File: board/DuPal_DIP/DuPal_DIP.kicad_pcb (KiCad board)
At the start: 2 copper layers, 113 x 78.7 mm, 57 parts, among them J1 AVR-ISP-6, J2 RS232, J3 Power IN, SW1 SW_Push, SW2 Power, U1 ATmega8A-PU, U10 24 Pin PAL, U2 74HC595, U3 74HC595, U5 20 Pin PAL, U6 MAX232, U7 L7805, U8 74HC166, U9 74HC595, Y1 8Mhz

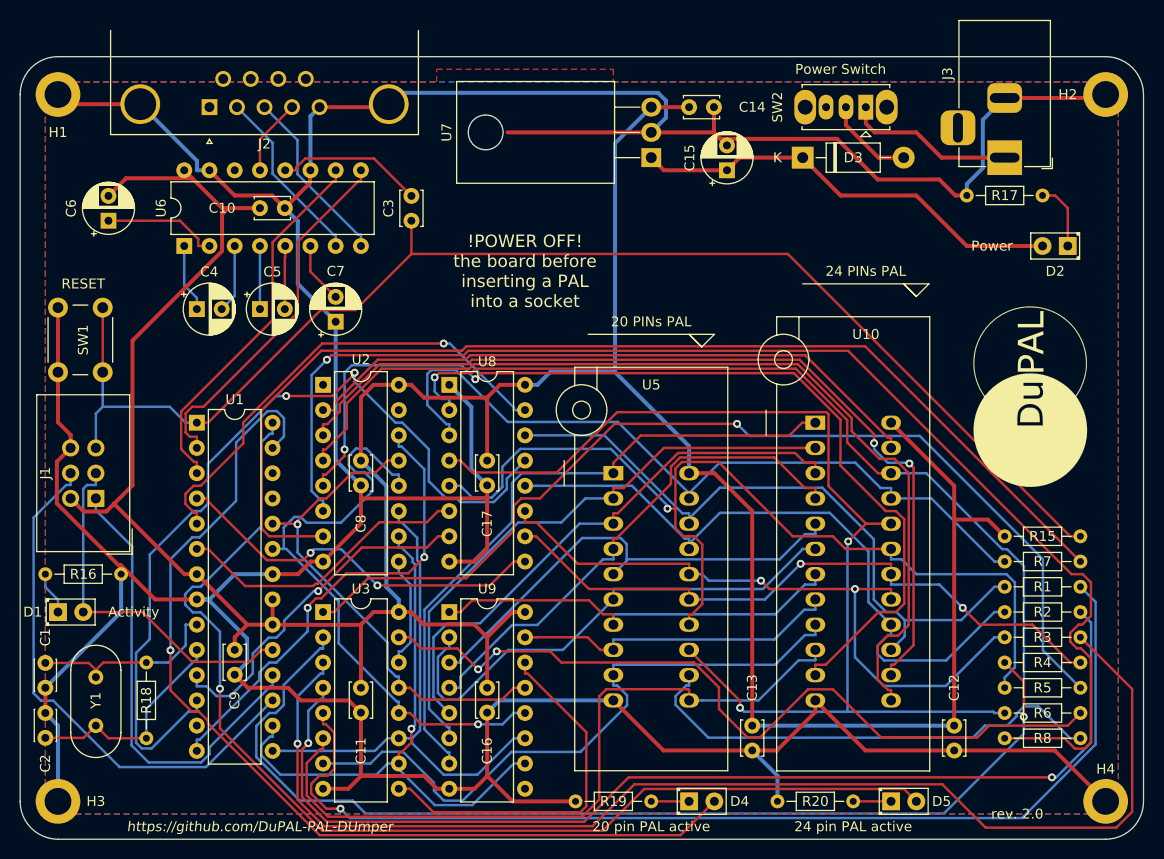
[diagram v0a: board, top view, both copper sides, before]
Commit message: Updated to KiCad 7
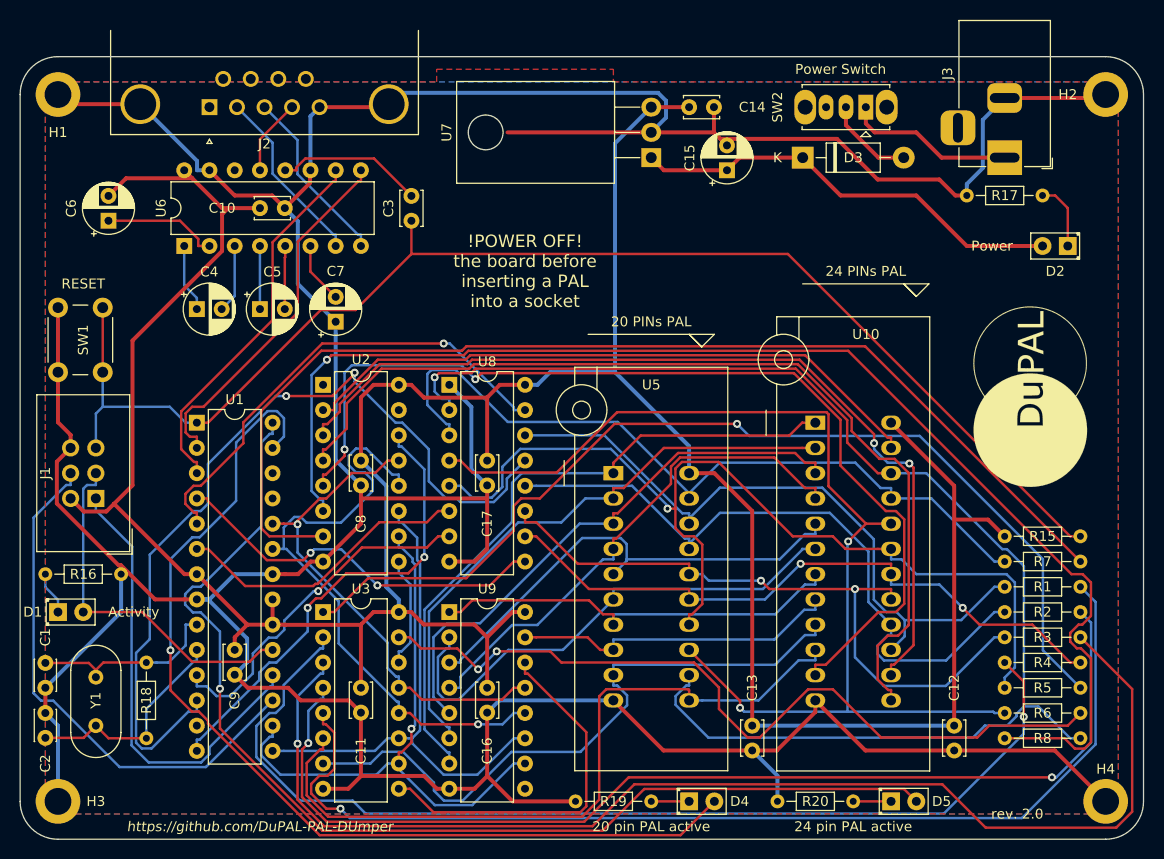
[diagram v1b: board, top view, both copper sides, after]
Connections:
- net /~PISO_CLR renamed /~{PISO_CLR}
- net /~RESET renamed /~{RESET}
- net /~SIPO_CLR renamed /~{SIPO_CLR}
- net /~SIPO_OE renamed /~{SIPO_OE}
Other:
- net class Default removed
- net class POWER removed
